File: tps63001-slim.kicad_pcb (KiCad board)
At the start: 2 copper layers, 15.7 x 15.7 mm, 10 parts, among them J1 Conn_01x04_Male, U1 TPS63001

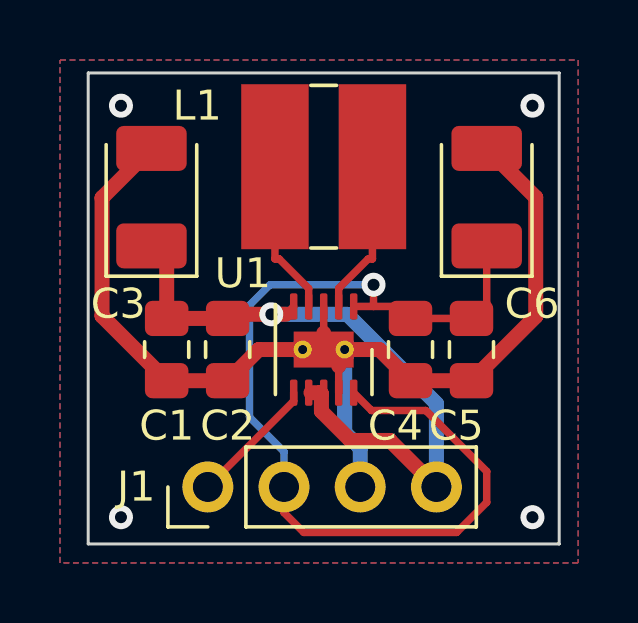
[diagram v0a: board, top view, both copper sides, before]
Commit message: single gerber
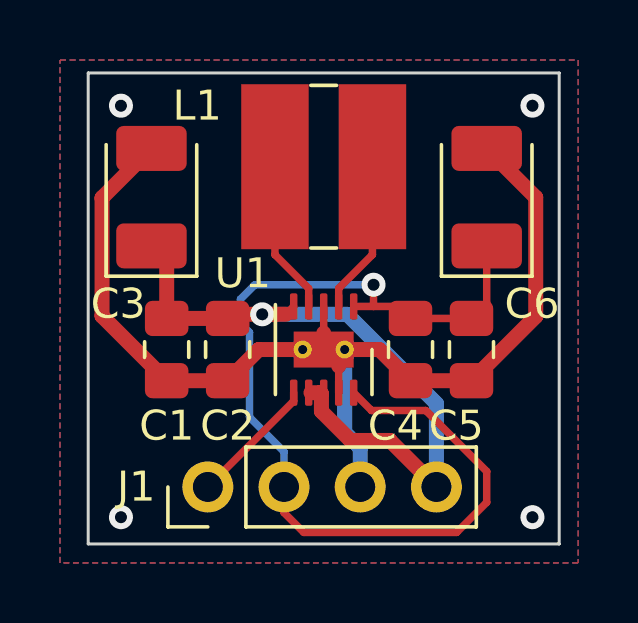
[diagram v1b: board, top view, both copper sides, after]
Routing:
- net Net-(C4-Pad1): track 33.2 -> 33.8 mm
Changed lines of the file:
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@@
     (fp_line (start 1.75 -1.4) (end -1.05 -1.4) (layer "F.Fab") (width 0.1))
     (fp_line (start 1.75 1.4) (end 1.75 -1.4) (layer "F.Fab") (width 0.1))
-    (pad "1" smd roundrect (at -1.625 0 90) (size 1.5 2.35) (layers "F.Cu" "F.Paste" "F.Mask") (roundrect_rratio 0.166667)
+    (pad "1" smd roundrect (at -1.625 0 90) (size 1.5 2.35) (layers "F.Cu" "F.Paste" "F.Mask") (roundrect_rratio 0.1666673333)
       (net 6 "Net-(C4-Pad1)") (pintype "passive"))
-    (pad "2" smd roundrect (at 1.625 0 90) (size 1.5 2.35) (layers "F.Cu" "F.Paste" "F.Mask") (roundrect_rratio 0.166667)
+    (pad "2" smd roundrect (at 1.625 0 90) (size 1.5 2.35) (layers "F.Cu" "F.Paste" "F.Mask") (roundrect_rratio 0.1666673333)
       (net 2 "Earth") (pintype "passive"))
     (model "${KICAD6_3DMODEL_DIR}/Capacitor_Tantalum_SMD.3dshapes/CP_EIA-3528-21_Kemet-B.wrl"
@@
     (fp_line (start -1.75 1.4) (end 1.75 1.4) (layer "F.Fab") (width 0.1))
     (fp_line (start -1.05 -1.4) (end -1.75 -0.7) (layer "F.Fab") (width 0.1))
-    (pad "1" smd roundrect (at -1.625 0 90) (size 1.5 2.35) (layers "F.Cu" "F.Paste" "F.Mask") (roundrect_rratio 0.166667)
+    (pad "1" smd roundrect (at -1.625 0 90) (size 1.5 2.35) (layers "F.Cu" "F.Paste" "F.Mask") (roundrect_rratio 0.1666673333)
       (net 1 "Net-(C1-Pad1)") (pintype "passive"))
-    (pad "2" smd roundrect (at 1.625 0 90) (size 1.5 2.35) (layers "F.Cu" "F.Paste" "F.Mask") (roundrect_rratio 0.166667)
+    (pad "2" smd roundrect (at 1.625 0 90) (size 1.5 2.35) (layers "F.Cu" "F.Paste" "F.Mask") (roundrect_rratio 0.1666673333)
       (net 2 "Earth") (pintype "passive"))
     (model "${KICAD6_3DMODEL_DIR}/Capacitor_Tantalum_SMD.3dshapes/CP_EIA-3528-21_Kemet-B.wrl"
@@
   (segment (start 107.8122 110.6953) (end 107.7744 110.6953) (width 0.2502) (layer "F.Cu") (net 1))
   (segment (start 107.7744 110.6953) (end 107.7366 110.6575) (width 0.5) (layer "F.Cu") (net 1))
-  (via (at 106.104 108.0446) (size 0.8) (drill 0.4) (layers "F.Cu" "B.Cu") (net 1))
+  (via (at 105.8 108.0446) (size 0.8) (drill 0.4) (layers "F.Cu" "B.Cu") (net 1))
   (segment (start 111.607 113.8) (end 111.607 111.019) (width 0.5) (layer "B.Cu") (net 1))
   (segment (start 111.607 111.019) (end 108.6326 108.0446) (width 0.5) (layer "B.Cu") (net 1))
@@
   (segment (start 108.55 109.22) (end 108.55 111.9827) (width 0.5) (layer "B.Cu") (net 2))
   (segment (start 107.85 109.22) (end 108.55 109.22) (width 0.5) (layer "B.Cu") (net 2))
-  (segment (start 106.225 106.1993) (end 106.3657 106.1993) (width 0.25) (layer "F.Cu") (net 3))
+  (segment (start 106.225 103.124) (end 106.225 106.0586) (width 0.25) (layer "F.Cu") (net 3))
+  (segment (start 106.225 106.0586) (end 107.35 107.1836) (width 0.25) (layer "F.Cu") (net 3))
   (segment (start 107.35 107.1836) (end 107.35 107.7825) (width 0.25) (layer "F.Cu") (net 3))
-  (segment (start 106.225 103.124) (end 106.225 106.1993) (width 0.25) (layer "F.Cu") (net 3))
-  (segment (start 106.3657 106.1993) (end 107.35 107.1836) (width 0.25) (layer "F.Cu") (net 3))
   (segment (start 103.987 113.8) (end 106.85 110.937) (width 0.25) (layer "F.Cu") (net 4))
   (segment (start 106.85 110.937) (end 106.85 110.6575) (width 0.25) (layer "F.Cu") (net 4))
-  (segment (start 109.475 103.124) (end 109.475 106.1993) (width 0.25) (layer "F.Cu") (net 5))
-  (segment (start 109.475 106.1993) (end 109.3343 106.1993) (width 0.25) (layer "F.Cu") (net 5))
+  (segment (start 109.475 106.0586) (end 108.35 107.1836) (width 0.25) (layer "F.Cu") (net 5))
+  (segment (start 109.475 103.124) (end 109.475 106.0586) (width 0.25) (layer "F.Cu") (net 5))
   (segment (start 108.35 107.1836) (end 108.35 107.7825) (width 0.25) (layer "F.Cu") (net 5))
-  (segment (start 109.3343 106.1993) (end 108.35 107.1836) (width 0.25) (layer "F.Cu") (net 5))
   (segment (start 113.284 105.765) (end 113.284 107.6745) (width 0.25) (layer "F.Cu") (net 6))
   (segment (start 110.344 107.7825) (end 109.5116 107.7825) (width 0.25) (layer "F.Cu") (net 6))
@@
   (via (at 109.5116 107.0594) (size 0.8) (drill 0.4) (layers "F.Cu" "B.Cu") (net 6))
   (segment (start 106.527 112.6247) (end 105.3764 111.4741) (width 0.25) (layer "B.Cu") (net 6))
-  (segment (start 105.3764 111.4741) (end 105.3764 107.744) (width 0.25) (layer "B.Cu") (net 6))
+  (segment (start 105.555424 107.0594) (end 109.5116 107.0594) (width 0.25) (layer "B.Cu") (net 6))
+  (segment (start 105.075 108.344905) (end 105.075 107.539824) (width 0.25) (layer "B.Cu") (net 6))
+  (segment (start 105.3764 108.646305) (end 105.075 108.344905) (width 0.25) (layer "B.Cu") (net 6))
+  (segment (start 105.075 107.539824) (end 105.555424 107.0594) (width 0.25) (layer "B.Cu") (net 6))
+  (segment (start 105.3764 111.4741) (end 105.3764 108.646305) (width 0.25) (layer "B.Cu") (net 6))
   (segment (start 106.527 113.8) (end 106.527 112.6247) (width 0.25) (layer "B.Cu") (net 6))
-  (segment (start 106.061 107.0594) (end 109.5116 107.0594) (width 0.25) (layer "B.Cu") (net 6))
-  (segment (start 105.3764 107.744) (end 106.061 107.0594) (width 0.25) (layer "B.Cu") (net 6))
   (zone (net 2) (net_name "Earth") (layers F&B.Cu) (hatch edge 0.508)
     (connect_pads (clearance 0.508))
